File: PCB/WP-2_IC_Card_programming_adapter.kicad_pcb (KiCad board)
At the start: 2 copper layers, 17.8 x 49.5 mm, 4 parts, among them J1 Conn_01x38_Male, J2 Conn_02x16_Counter_Clockwise, J3 Conn_02x08_Odd_Even

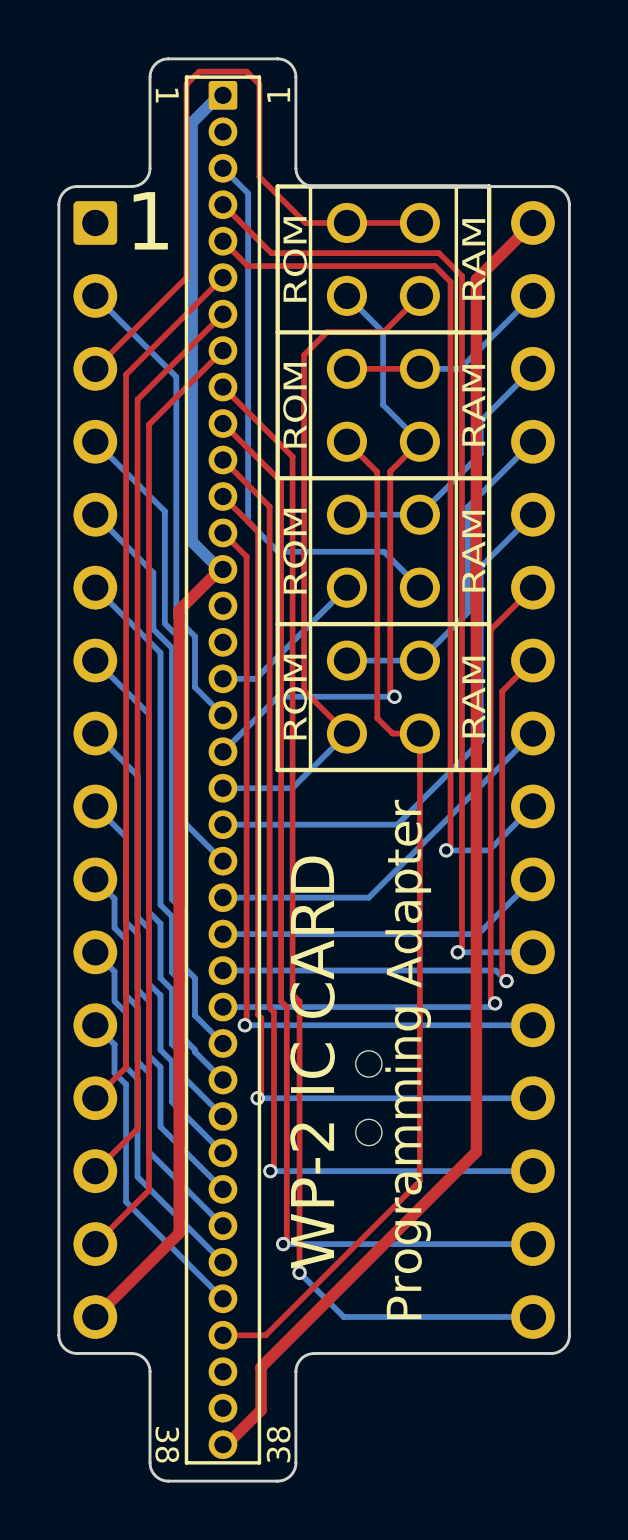
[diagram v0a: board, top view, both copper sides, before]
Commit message: kicad 6
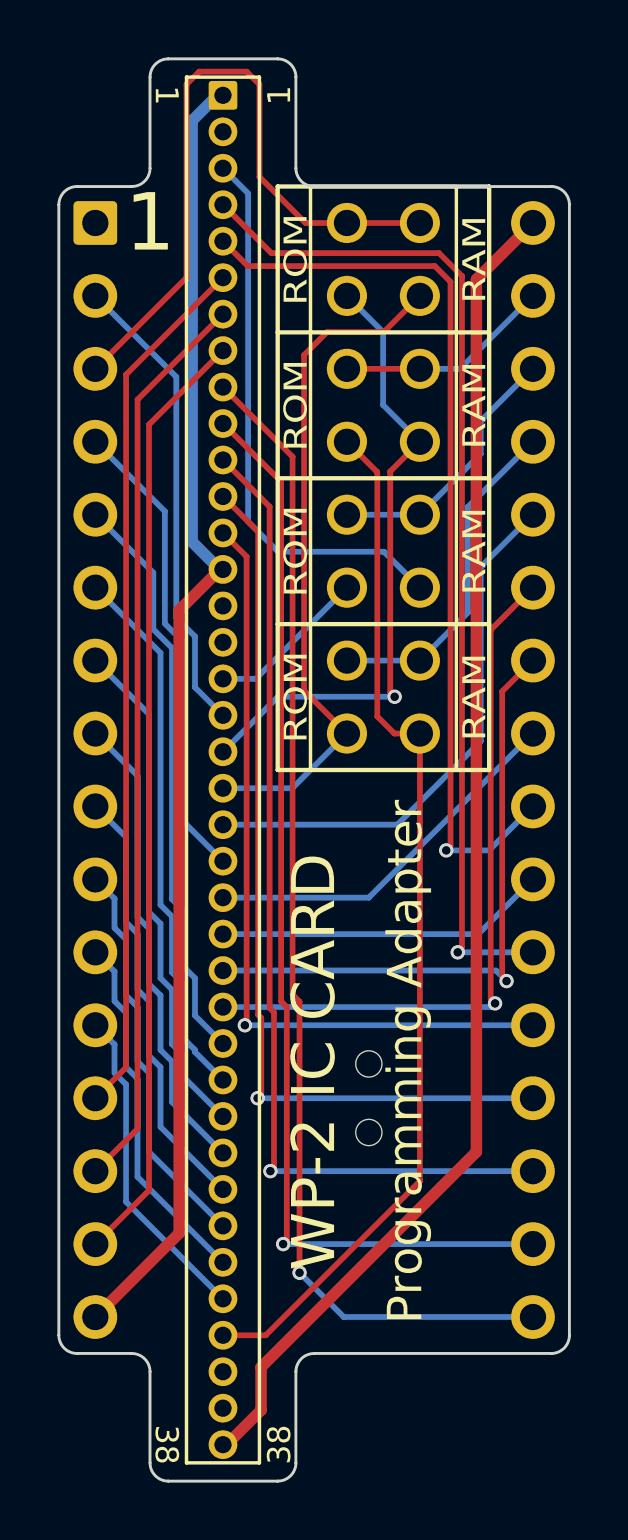
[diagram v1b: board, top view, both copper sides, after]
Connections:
- net /A14_~WE renamed /A14_~{WE}
- net /R~W renamed /R~{W}
- net /~CE1 renamed /~{CE1}
- net /~OE renamed /~{OE}
- net /~WE~_A15 renamed /~{WE}_A15
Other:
- net class Default removed
